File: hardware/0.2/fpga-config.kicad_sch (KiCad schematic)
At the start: 30 parts, among them J2 JTAG, J5 USB_C_Receptacle_USB2.0, Q1 BSS138, SW1 PTS810, U1 ECP5U_12_CABGA256, U4 USBLC6-2P6, U6 W25Q128JVPIQ

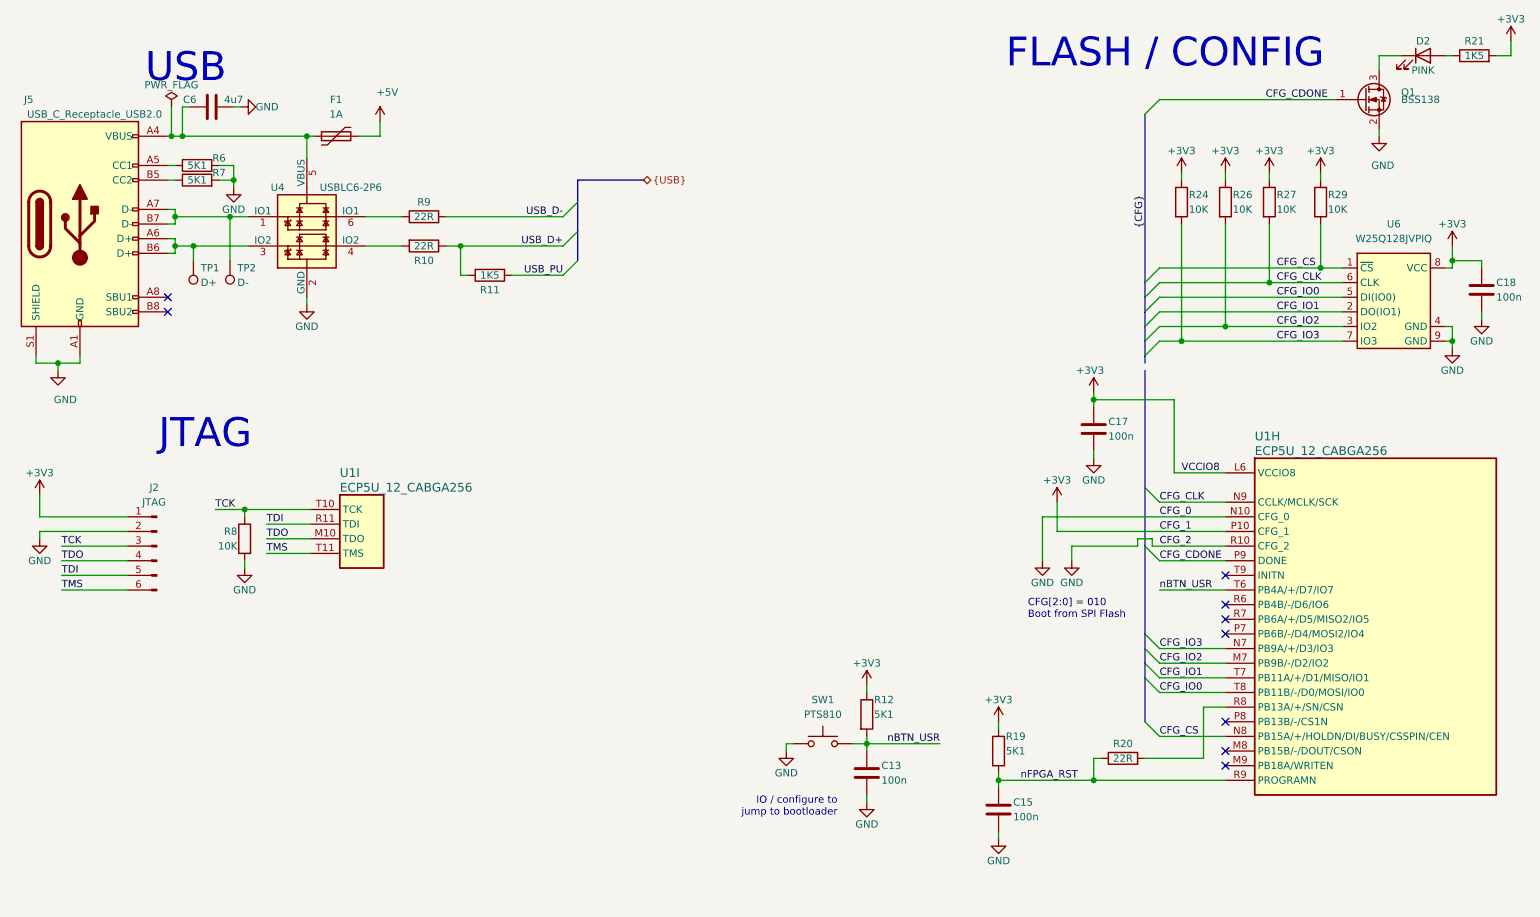
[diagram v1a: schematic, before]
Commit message: almost there
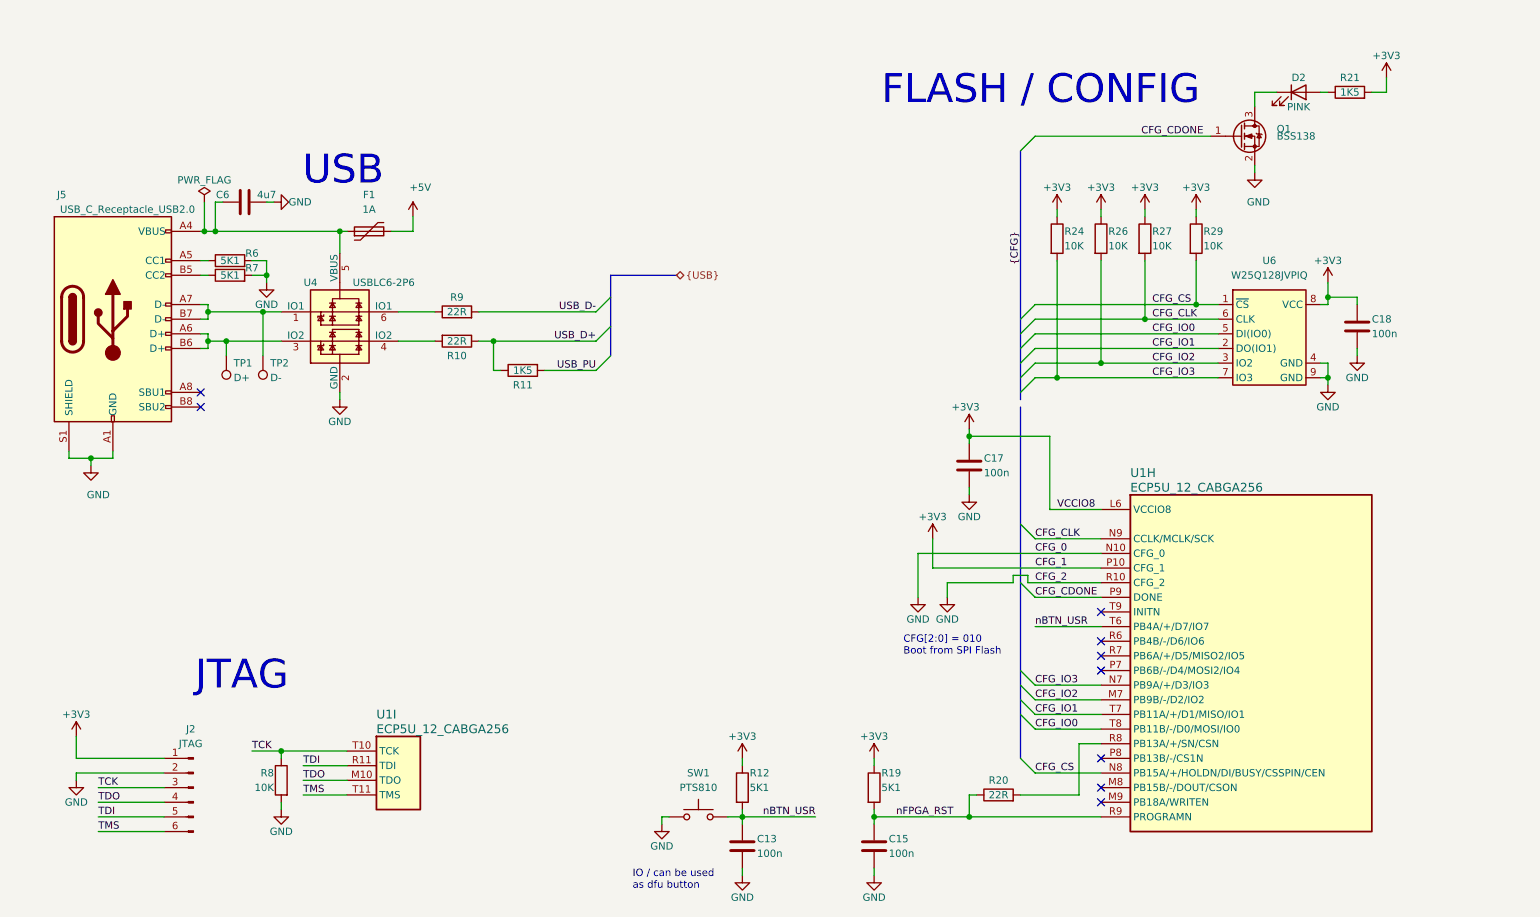
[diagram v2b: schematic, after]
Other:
- note added: "IO / can be used as dfu button"
- note removed: "IO / configure to jump to bootloader"
- moved on the sheet: C13, C15, C17, C18, C6, D2, F1, J2, J5, Q1, R10, R11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
